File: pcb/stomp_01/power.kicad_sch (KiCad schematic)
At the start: 14 parts, among them J11 Barrel_Jack, U2 TPS54331DR

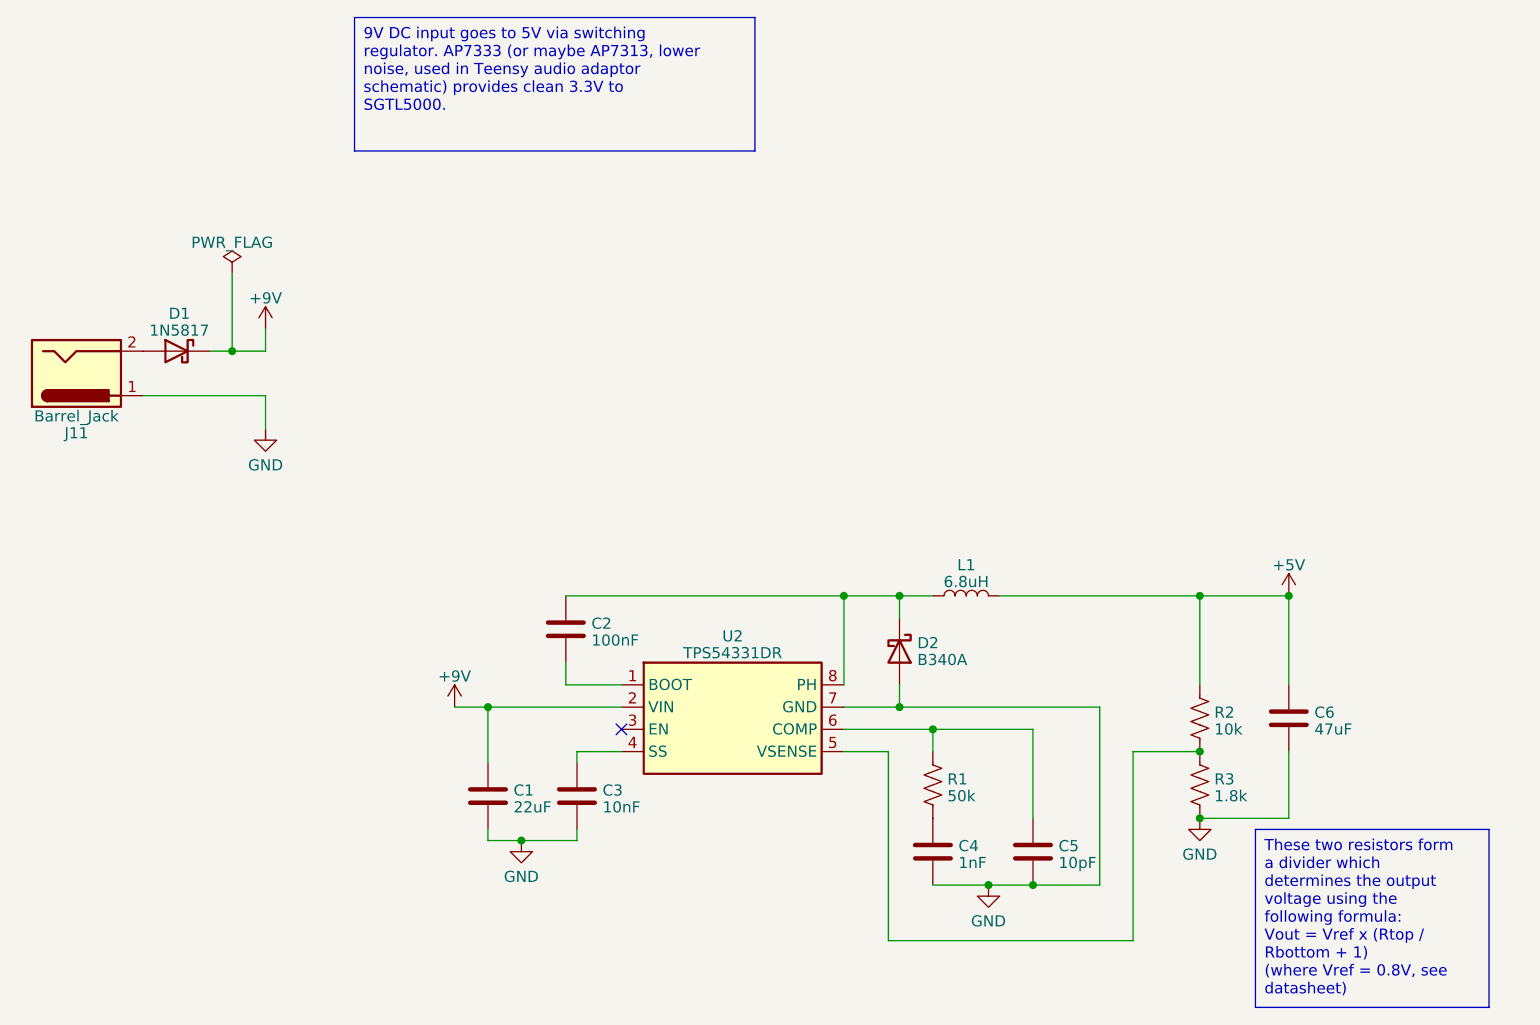
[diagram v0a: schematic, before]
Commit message: looking nice
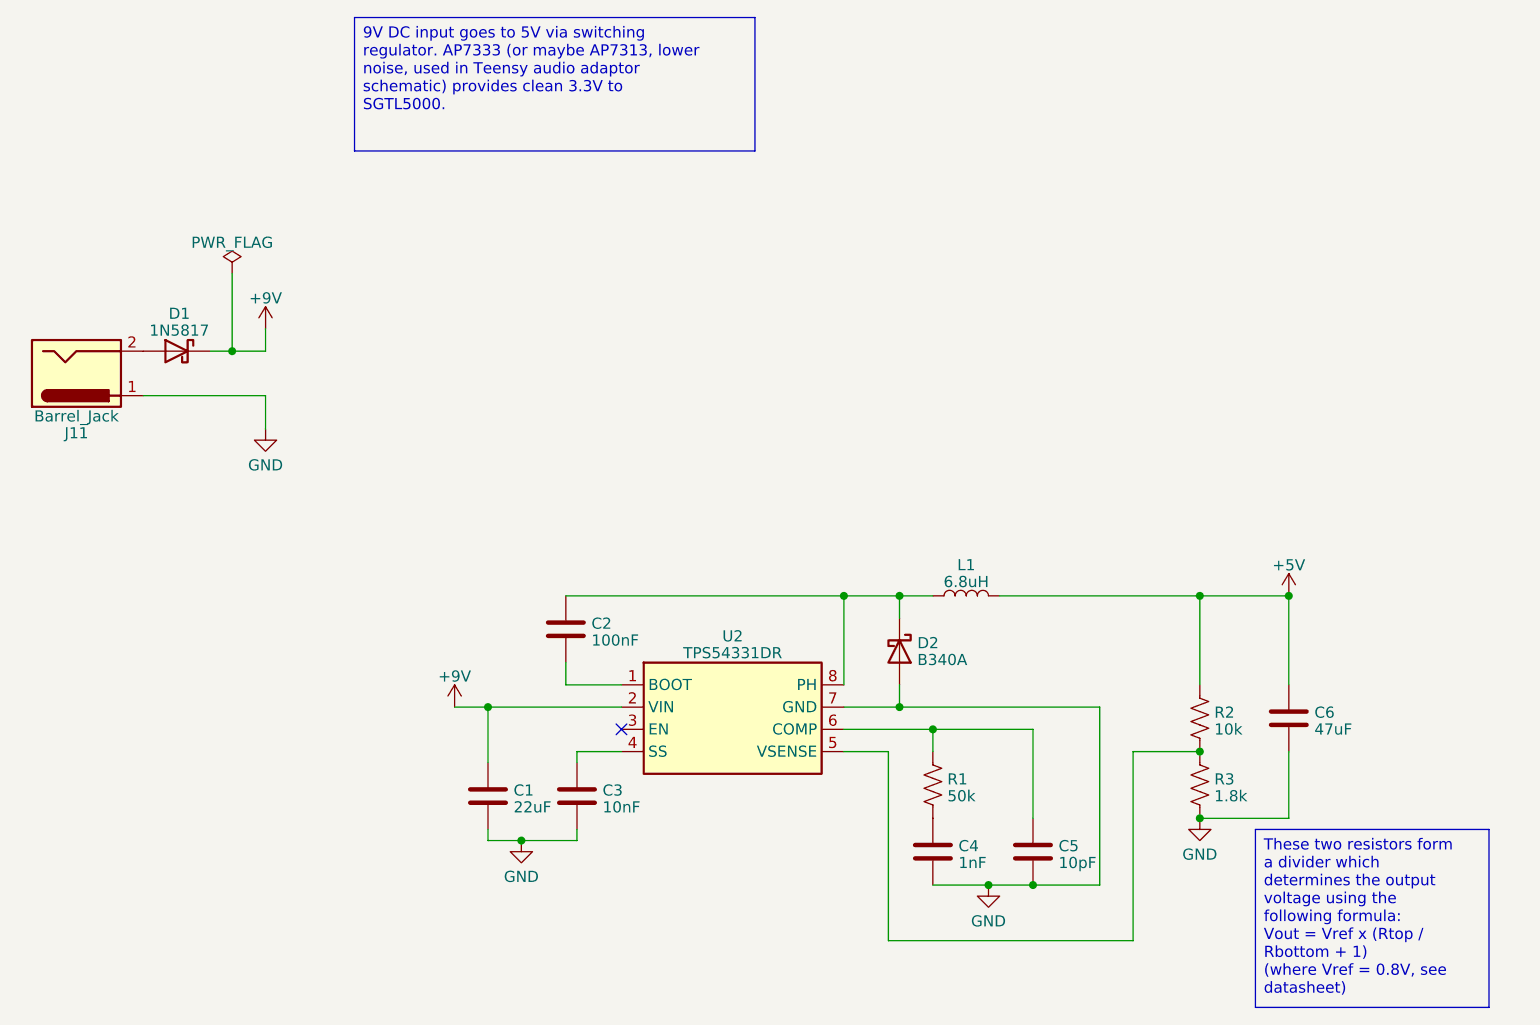
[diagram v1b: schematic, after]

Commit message: pre routing
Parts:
- J11: footprint Connector_PinHeader_2.54mm:PinHeader_1x02_P2.54mm_Vertical -> Connector_Wire:SolderWire-1sqmm_1x02_P5.4mm_D1.4mm_OD2.7mm
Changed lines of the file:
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@@
 			)
 		)
-		(property "Footprint" "Connector_PinHeader_2.54mm:PinHeader_1x02_P2.54mm_Vertical"
+		(property "Footprint" "Connector_Wire:SolderWire-1sqmm_1x02_P5.4mm_D1.4mm_OD2.7mm"
 			(at 58.42 58.674 0)
 			(effects
